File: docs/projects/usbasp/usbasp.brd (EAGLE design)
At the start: 84.8 x 50.8 mm, 29 parts, among them Q1 12MHz

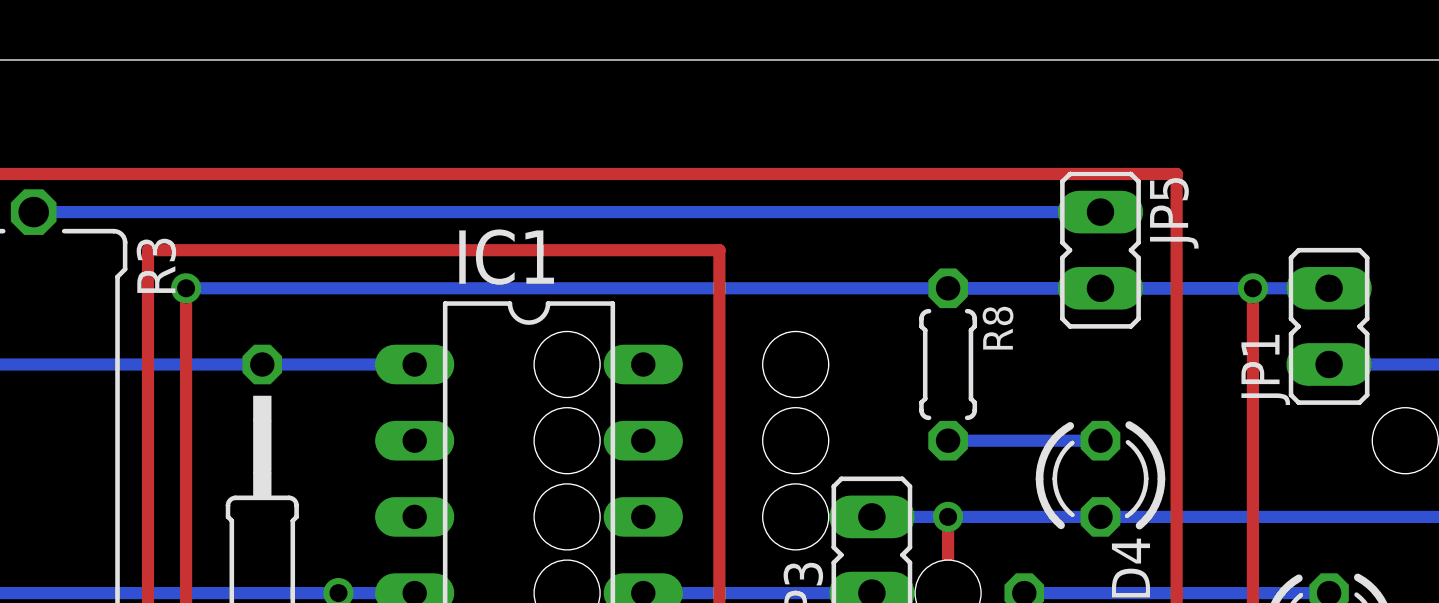
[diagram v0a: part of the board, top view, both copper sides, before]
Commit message: fix airwires
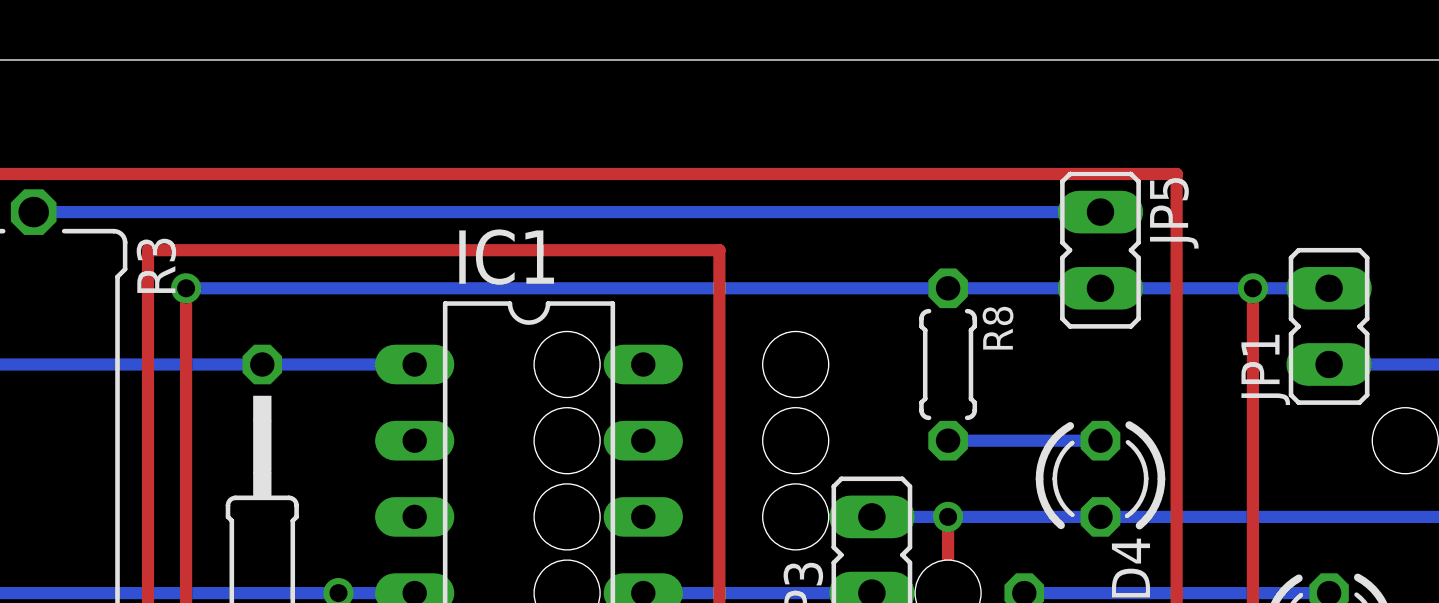
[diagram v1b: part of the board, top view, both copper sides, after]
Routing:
- net N$3: track 135.0 -> 124.8 mm
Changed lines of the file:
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@@
 <wire x1="60.96" y1="17.78" x2="53.34" y2="17.78" width="0.4064" layer="16"/>
 <wire x1="73.66" y1="17.78" x2="68.58" y2="17.78" width="0.4064" layer="16"/>
-<wire x1="73.66" y1="40.64" x2="63.5" y2="40.64" width="0.4064" layer="16"/>
 <wire x1="73.66" y1="40.64" x2="76.2" y2="40.64" width="0.4064" layer="16"/>
-<wire x1="38.1" y1="40.64" x2="73.66" y2="40.64" width="0.4064" layer="16"/>
+<wire x1="38.1" y1="40.64" x2="63.5" y2="40.64" width="0.4064" layer="16"/>
+<wire x1="68.58" y1="40.64" x2="73.66" y2="40.64" width="0.4064" layer="16"/>
 <wire x1="38.1" y1="22.86" x2="38.1" y2="40.64" width="0.4064" layer="1"/>
 <wire x1="22.49" y1="22.88" x2="25.4" y2="22.88" width="0.4064" layer="16"/>
 <wire x1="25.4" y1="22.88" x2="25.4" y2="22.86" width="0.4064" layer="16"/>
 <wire x1="25.4" y1="22.86" x2="38.1" y2="22.86" width="0.4064" layer="16"/>
-<wire x1="63.5" y1="40.64" x2="68.58" y2="40.64" width="0" layer="19" extent="1-1"/>
 <via x="38.1" y="22.86" extent="1-16" drill="0.6" shape="square"/>
 <via x="73.66" y="17.78" extent="1-16" drill="0.6" shape="square"/>
 <via x="73.66" y="40.64" extent="1-16" drill="0.6" shape="square"/>
 <via x="38.1" y="40.64" extent="1-16" drill="0.6" shape="square"/>
+<wire x1="63.5" y1="40.64" x2="68.58" y2="40.64" width="0.4064" layer="16"/>
 </signal>
 <signal name="N$6">
